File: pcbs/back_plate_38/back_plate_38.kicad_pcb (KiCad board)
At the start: 2 copper layers, 117.6 x 95.3 mm, 6 parts

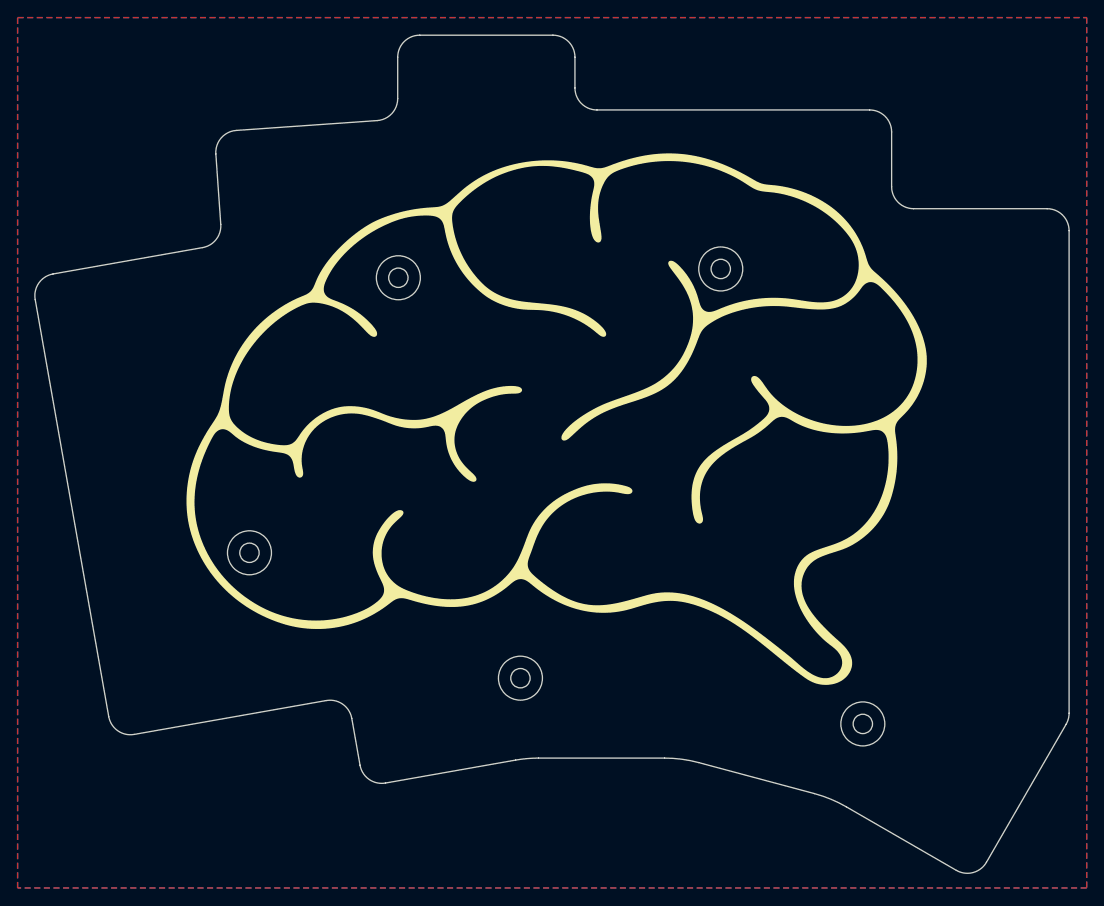
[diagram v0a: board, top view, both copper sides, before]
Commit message: update generated files
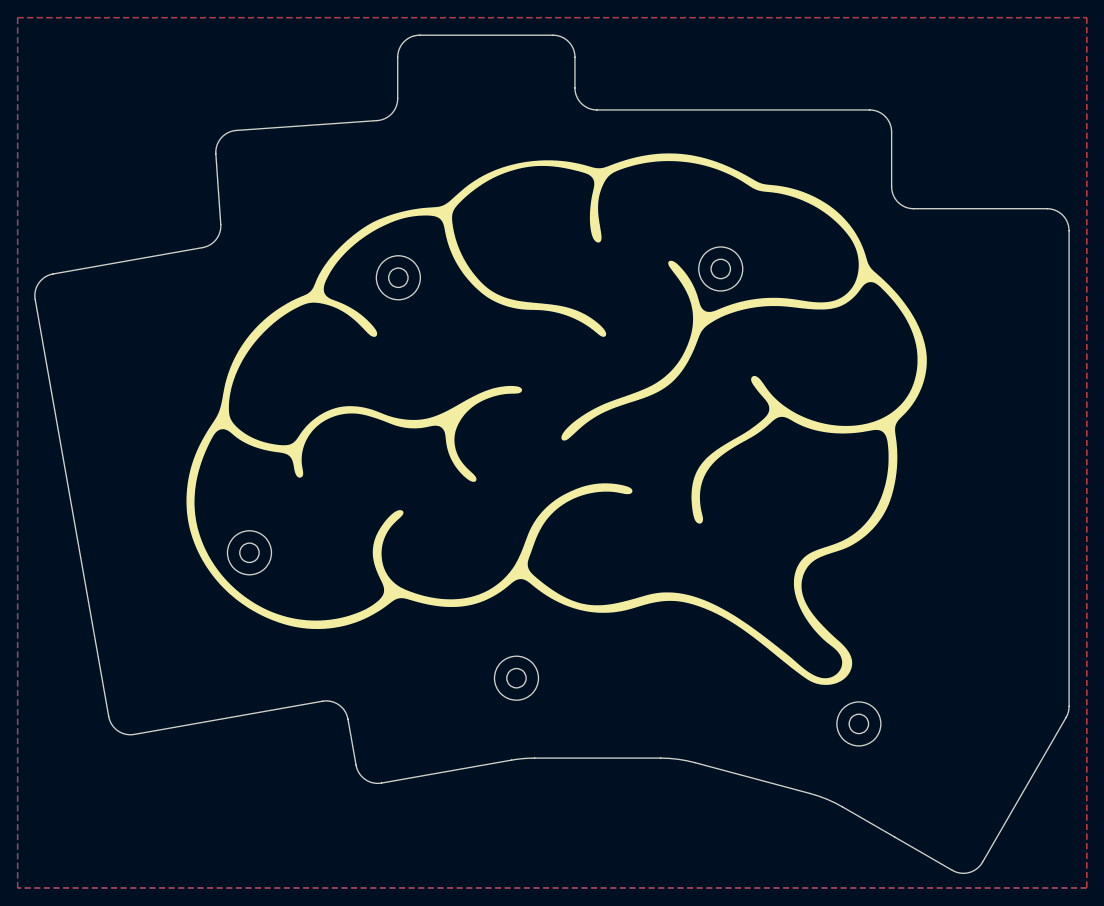
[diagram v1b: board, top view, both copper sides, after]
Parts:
- moved MH3 0.45 mm to (142.8, 97.7)
- moved MH4 0.45 mm to (103.9, 92.5)
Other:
- outline, holes or cut-outs redrawn
